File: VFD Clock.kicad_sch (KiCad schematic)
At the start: 33 parts, among them J2 Mode Button, J3 Up Button, J4 Down Button, J5 Select Button, U1 74HC595, U10 74HC595, U11 UDN2981A, U12 Minute Right, U13 74HC595, U14 UDN2981A, U15 Second Left, U16 74HC595, U17 UDN2981A, U18 Second Right, U19 XL6009 Module, U2 UDN2981A, U20 LM2596 Module, U21 DS3231 Module, U3 Hour Left, U4 74HC595, U5 UDN2981A, U6 Hour Right, U7 74HC595, U8 UDN2981A, U9 Minute Left

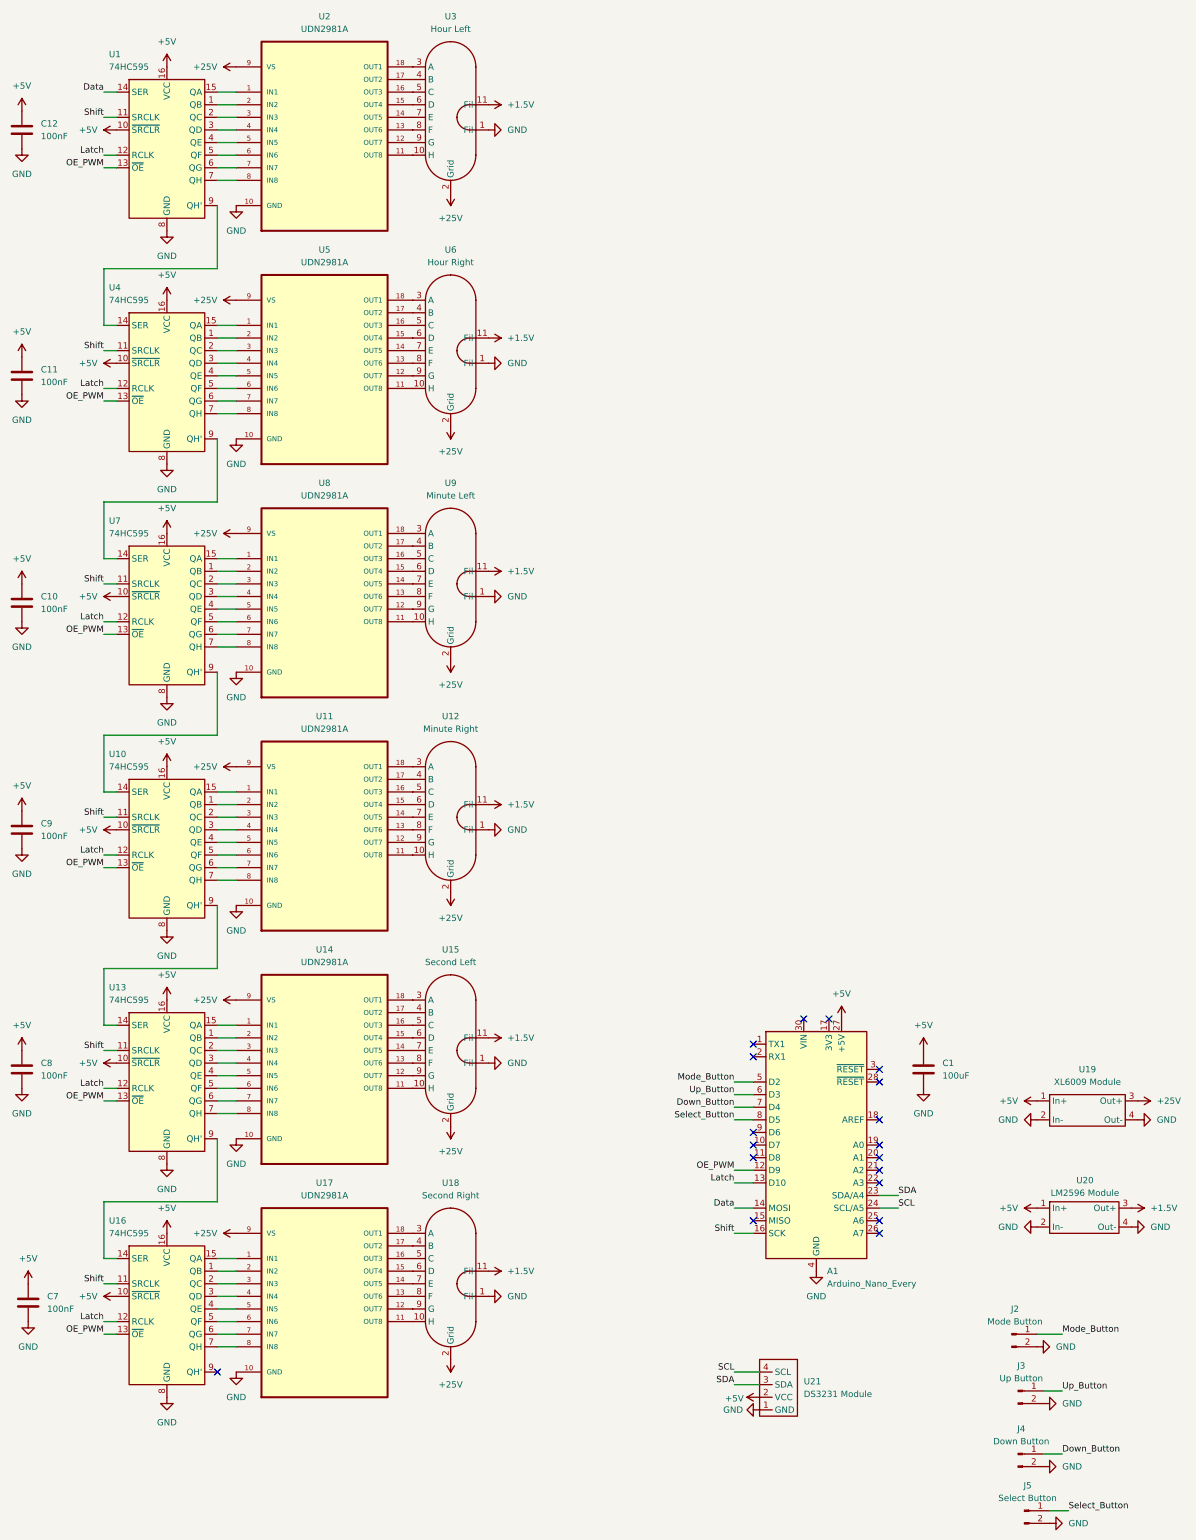
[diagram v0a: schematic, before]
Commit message: save
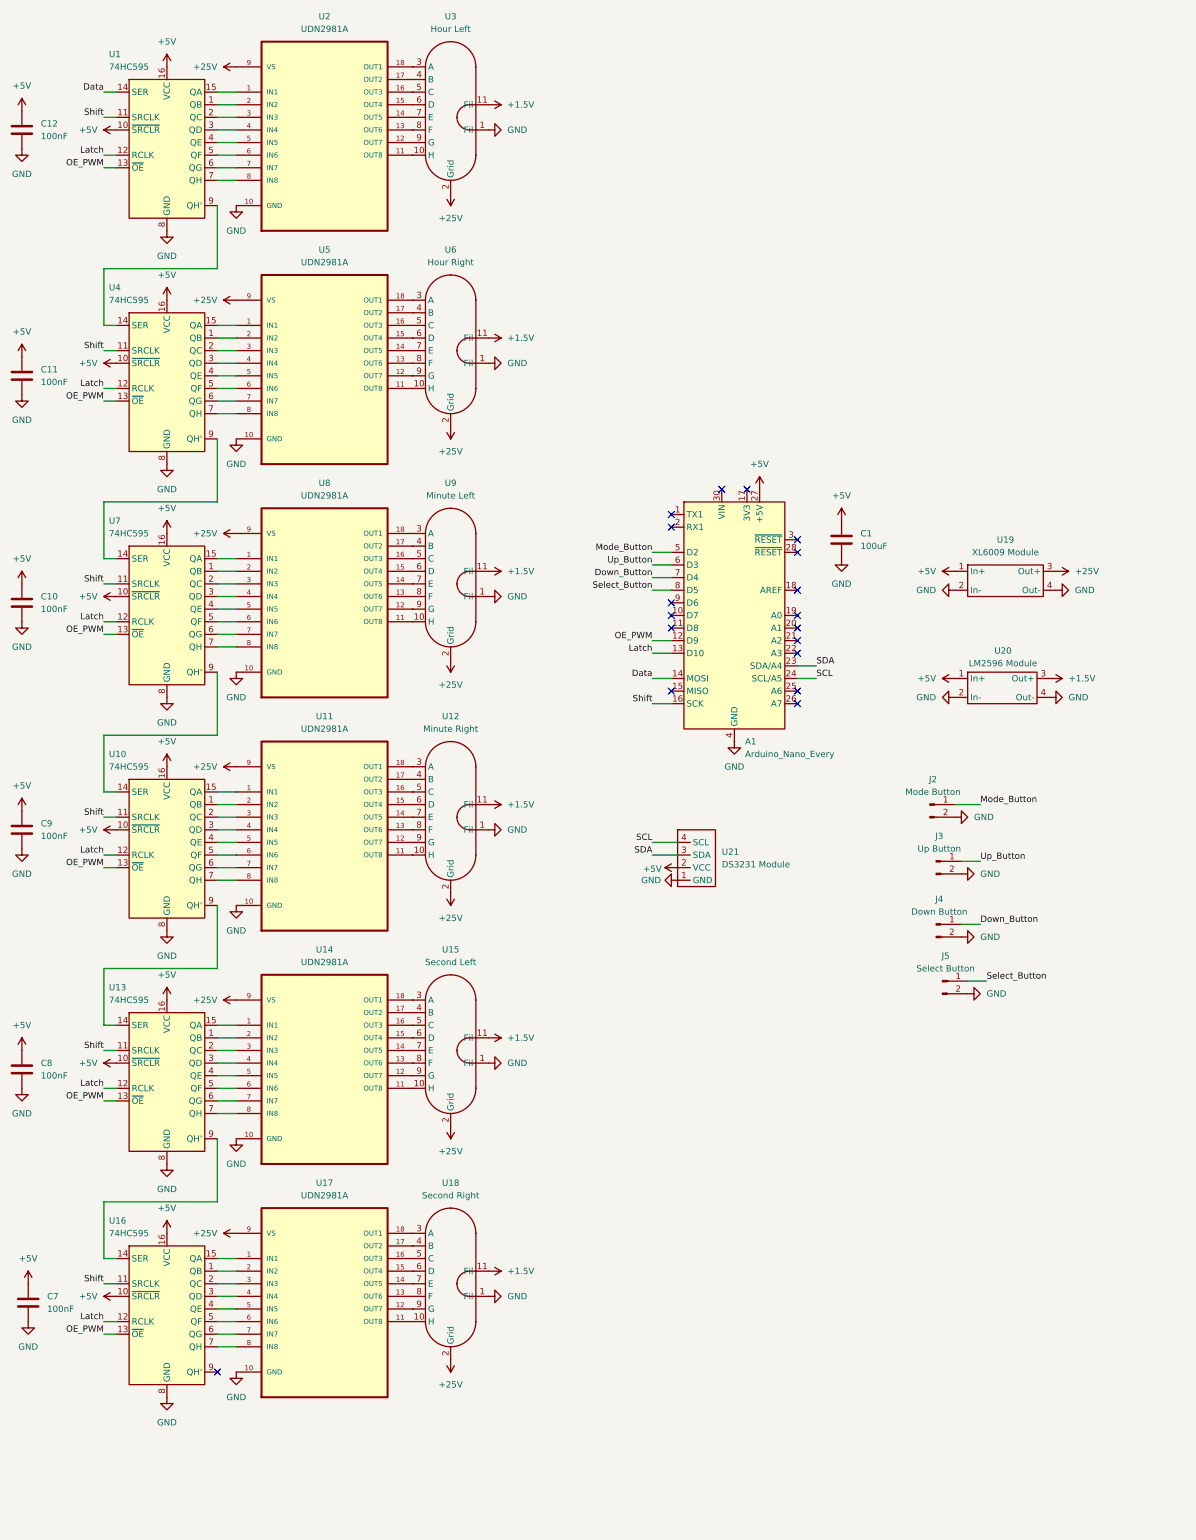
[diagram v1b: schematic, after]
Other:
- moved on the sheet: A1, C1, J2, J3, J4, J5, U19, U20, U21
